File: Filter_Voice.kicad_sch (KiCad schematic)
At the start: 25 parts, among them U3 TL072, U4 SSI2144

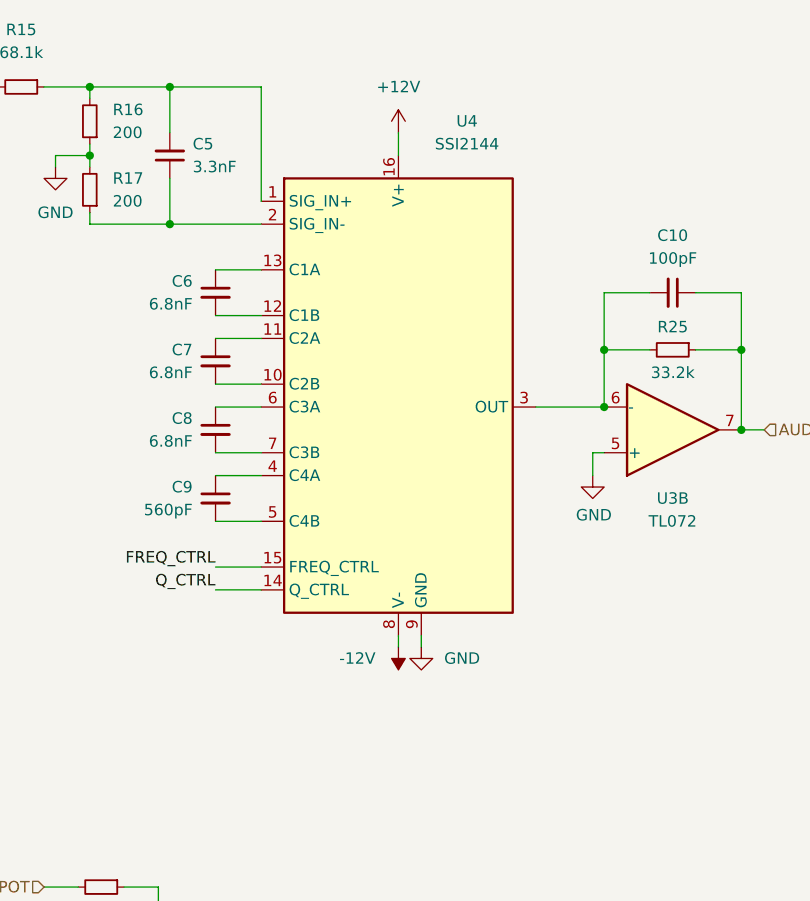
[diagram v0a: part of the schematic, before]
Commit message: First draft of component PCB routed
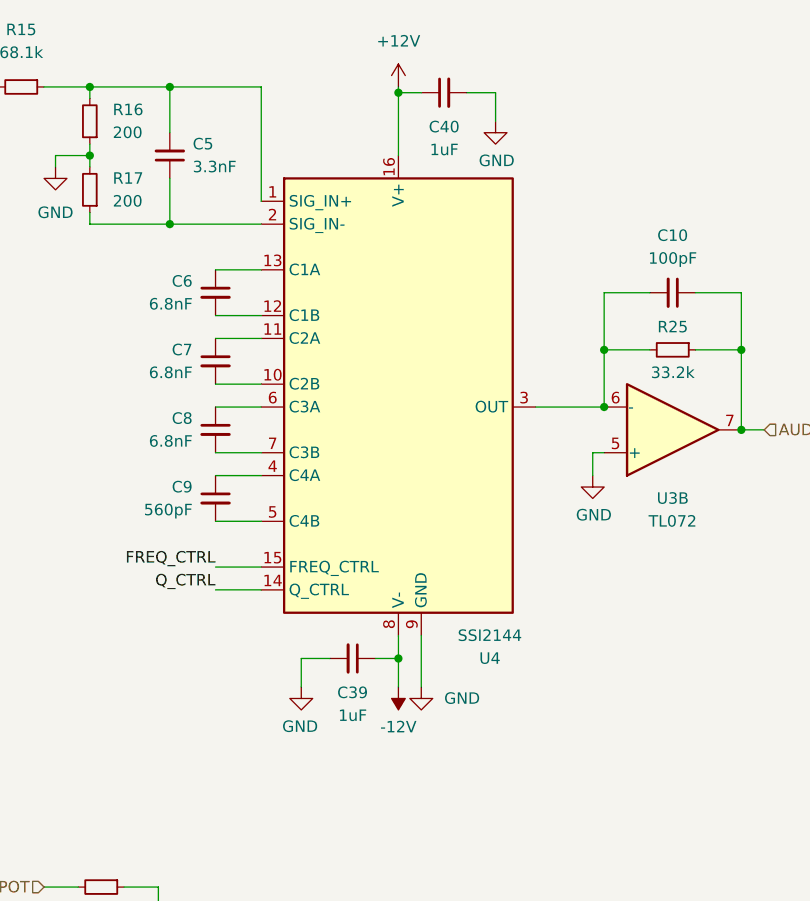
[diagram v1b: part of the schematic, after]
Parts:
- added C39, C40: 1uF, Capacitor_SMD:C_0603_1608Metric_Pad1.08x0.95mm_HandSolder, symbol Device:C_Small
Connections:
- net +12V: now also C40.1
- net -12V: now also C39.1
- net GND: now also C39.2, C40.2
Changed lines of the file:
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@@
   (junction (at 92.71 138.43) (diameter 0) (color 0 0 0 0)
   )
+  (junction (at 80.01 29.845) (diameter 0) (color 0 0 0 0)
+  )
   (junction (at 69.85 128.27) (diameter 0) (color 0 0 0 0)
   )
@@
   (junction (at 158.75 72.39) (diameter 0) (color 0 0 0 0)
   )
+  (junction (at 80.01 92.71) (diameter 0) (color 0 0 0 0)
+  )
   (junction (at 53.34 128.27) (diameter 0) (color 0 0 0 0)
   )
@@
     (stroke (width 0) (type default) (color 0 0 0 0))
   )
+  (wire (pts (xy 82.55 29.845) (xy 80.01 29.845))
+    (stroke (width 0) (type default) (color 0 0 0 0))
+  )
   (wire (pts (xy 45.72 36.83) (xy 45.72 38.1))
     (stroke (width 0) (type default) (color 0 0 0 0))
@@
     (stroke (width 0) (type default) (color 0 0 0 0))
   )
+  (wire (pts (xy 72.39 92.71) (xy 69.215 92.71))
+    (stroke (width 0) (type default) (color 0 0 0 0))
+  )
   (wire (pts (xy 40.64 128.27) (xy 44.45 128.27))
     (stroke (width 0) (type default) (color 0 0 0 0))
@@
     (stroke (width 0) (type default) (color 0 0 0 0))
   )
-  (wire (pts (xy 82.55 91.44) (xy 82.55 90.17))
-    (stroke (width 0) (type default) (color 0 0 0 0))
-  )
-  (wire (pts (xy 80.01 91.44) (xy 80.01 90.17))
+  (wire (pts (xy 82.55 95.885) (xy 82.55 90.17))
+    (stroke (width 0) (type default) (color 0 0 0 0))
+  )
+  (wire (pts (xy 80.01 95.885) (xy 80.01 92.71))
+    (stroke (width 0) (type default) (color 0 0 0 0))
+  )
+  (wire (pts (xy 77.47 92.71) (xy 80.01 92.71))
     (stroke (width 0) (type default) (color 0 0 0 0))
   )
@@
     (stroke (width 0) (type default) (color 0 0 0 0))
   )
+  (wire (pts (xy 90.805 29.845) (xy 90.805 33.02))
+    (stroke (width 0) (type default) (color 0 0 0 0))
+  )
   (wire (pts (xy 66.04 125.73) (xy 66.04 123.19))
     (stroke (width 0) (type default) (color 0 0 0 0))
@@
     (stroke (width 0) (type default) (color 0 0 0 0))
   )
+  (wire (pts (xy 69.215 92.71) (xy 69.215 95.885))
+    (stroke (width 0) (type default) (color 0 0 0 0))
+  )
   (wire (pts (xy 113.03 52.07) (xy 118.11 52.07))
     (stroke (width 0) (type default) (color 0 0 0 0))
@@
     (stroke (width 0) (type default) (color 0 0 0 0))
   )
+  (wire (pts (xy 87.63 29.845) (xy 90.805 29.845))
+    (stroke (width 0) (type default) (color 0 0 0 0))
+  )
   (wire (pts (xy 113.03 58.42) (xy 118.11 58.42))
     (stroke (width 0) (type default) (color 0 0 0 0))
@@
     (stroke (width 0) (type default) (color 0 0 0 0))
   )
+  (wire (pts (xy 80.01 92.71) (xy 80.01 90.17))
+    (stroke (width 0) (type default) (color 0 0 0 0))
+  )
   (wire (pts (xy 158.75 72.39) (xy 161.29 72.39))
     (stroke (width 0) (type default) (color 0 0 0 0))
@@
     (stroke (width 0) (type default) (color 0 0 0 0))
   )
-  (wire (pts (xy 80.01 36.83) (xy 80.01 34.29))
+  (wire (pts (xy 80.01 36.83) (xy 80.01 29.845))
     (stroke (width 0) (type default) (color 0 0 0 0))
   )
@@
   )
   (wire (pts (xy 69.85 128.27) (xy 69.85 138.43))
+    (stroke (width 0) (type default) (color 0 0 0 0))
+  )
+  (wire (pts (xy 80.01 29.845) (xy 80.01 29.21))
     (stroke (width 0) (type default) (color 0 0 0 0))
   )
@@
     (pin "3")
   )
+  (symbol (lib_id "power:GND") (at 69.215 95.885 0) (mirror y) (unit 1)
+    (in_bom yes) (on_board yes)
+    (property "Reference" "#PWR080" (id 0) (at 69.215 102.235 0)
+      (effects (font (size 1.27 1.27)) hide)
+    )
+    (property "Value" "GND" (id 1) (at 69.088 100.2792 0))
+    (property "Footprint" "" (id 2) (at 69.215 95.885 0)
+      (effects (font (size 1.27 1.27)) hide)
+    )
+    (property "Datasheet" "" (id 3) (at 69.215 95.885 0)
+      (effects (font (size 1.27 1.27)) hide)
+    )
+    (pin "1")
+  )
   (symbol (lib_id "Device:R_Small") (at 38.1 29.21 270) (unit 1)
     (in_bom yes) (on_board yes) (fields_autoplaced)
@@
     (pin "2")
   )
+  (symbol (lib_id "Device:C_Small") (at 85.09 29.845 90) (unit 1)
+    (in_bom yes) (on_board yes) (fields_autoplaced)
+    (property "Reference" "C40" (id 0) (at 85.0964 33.655 90))
+    (property "Value" "1uF" (id 1) (at 85.0964 36.195 90))
+    (property "Footprint" "Capacitor_SMD:C_0603_1608Metric_Pad1.08x0.95mm_HandSolder" (id 2) (at 85.09 29.845 0)
+      (effects (font (size 1.27 1.27)) hide)
+    )
+    (property "Datasheet" "~" (id 3) (at 85.09 29.845 0)
+      (effects (font (size 1.27 1.27)) hide)
+    )
+    (pin "1")
+    (pin "2")
+  )
   (symbol (lib_id "power:GND") (at 78.74 148.59 0) (unit 1)
     (in_bom yes) (on_board yes)
@@
     (pin "1")
   )
-  (symbol (lib_id "power:-12V") (at 80.01 91.44 180) (unit 1)
-    (in_bom yes) (on_board yes) (fields_autoplaced)
-    (property "Reference" "#PWR030" (id 0) (at 80.01 93.98 0)
-      (effects (font (size 1.27 1.27)) hide)
-    )
-    (property "Value" "-12V" (id 1) (at 77.47 92.7099 0)
-      (effects (font (size 1.27 1.27)) (justify left))
-    )
-    (property "Footprint" "" (id 2) (at 80.01 91.44 0)
-      (effects (font (size 1.27 1.27)) hide)
-    )
-    (property "Datasheet" "" (id 3) (at 80.01 91.44 0)
+  (symbol (lib_id "power:-12V") (at 80.01 95.885 180) (unit 1)
+    (in_bom yes) (on_board yes) (fields_autoplaced)
+    (property "Reference" "#PWR030" (id 0) (at 80.01 98.425 0)
+      (effects (font (size 1.27 1.27)) hide)
+    )
+    (property "Value" "-12V" (id 1) (at 80.01 100.33 0))
+    (property "Footprint" "" (id 2) (at 80.01 95.885 0)
+      (effects (font (size 1.27 1.27)) hide)
+    )
+    (property "Datasheet" "" (id 3) (at 80.01 95.885 0)
       (effects (font (size 1.27 1.27)) hide)
     )
@@
     (pin "2")
   )
+  (symbol (lib_id "power:GND") (at 90.805 33.02 0) (unit 1)
+    (in_bom yes) (on_board yes)
+    (property "Reference" "#PWR081" (id 0) (at 90.805 39.37 0)
+      (effects (font (size 1.27 1.27)) hide)
+    )
+    (property "Value" "GND" (id 1) (at 90.932 37.4142 0))
+    (property "Footprint" "" (id 2) (at 90.805 33.02 0)
+      (effects (font (size 1.27 1.27)) hide)
+    )
+    (property "Datasheet" "" (id 3) (at 90.805 33.02 0)
+      (effects (font (size 1.27 1.27)) hide)
+    )
+    (pin "1")
+  )
+  (symbol (lib_id "Device:C_Small") (at 74.93 92.71 270) (mirror x) (unit 1)
+    (in_bom yes) (on_board yes) (fields_autoplaced)
+    (property "Reference" "C39" (id 0) (at 74.9236 96.52 90))
+    (property "Value" "1uF" (id 1) (at 74.9236 99.06 90))
+    (property "Footprint" "Capacitor_SMD:C_0603_1608Metric_Pad1.08x0.95mm_HandSolder" (id 2) (at 74.93 92.71 0)
+      (effects (font (size 1.27 1.27)) hide)
+    )
+    (property "Datasheet" "~" (id 3) (at 74.93 92.71 0)
+      (effects (font (size 1.27 1.27)) hide)
+    )
+    (pin "1")
+    (pin "2")
+  )
   (symbol (lib_id "power:+12V") (at 90.17 148.59 90) (unit 1)
     (in_bom yes) (on_board yes)
@@
   (symbol (lib_id "Audio:SSI2144") (at 80.01 64.77 0) (unit 1)
     (in_bom yes) (on_board yes)
-    (property "Reference" "U4" (id 0) (at 87.63 33.02 0))
-    (property "Value" "SSI2144" (id 1) (at 87.63 35.56 0))
+    (property "Reference" "U4" (id 0) (at 90.17 92.71 0))
+    (property "Value" "SSI2144" (id 1) (at 90.17 90.17 0))
     (property "Footprint" "Package_SO:SSOP-16_3.9x4.9mm_P0.635mm" (id 2) (at 102.87 67.31 0)
       (effects (font (size 1.27 1.27)) hide)
@@
     (pin "2")
   )
-  (symbol (lib_id "power:+12V") (at 80.01 34.29 0) (unit 1)
-    (in_bom yes) (on_board yes) (fields_autoplaced)
-    (property "Reference" "#PWR029" (id 0) (at 80.01 38.1 0)
-      (effects (font (size 1.27 1.27)) hide)
-    )
-    (property "Value" "+12V" (id 1) (at 80.01 29.21 0))
-    (property "Footprint" "" (id 2) (at 80.01 34.29 0)
-      (effects (font (size 1.27 1.27)) hide)
-    )
-    (property "Datasheet" "" (id 3) (at 80.01 34.29 0)
-      (effects (font (size 1.27 1.27)) hide)
-    )
-    (pin "1")
-  )
-  (symbol (lib_id "power:GND") (at 82.55 91.44 0) (unit 1)
-    (in_bom yes) (on_board yes) (fields_autoplaced)
-    (property "Reference" "#PWR031" (id 0) (at 82.55 97.79 0)
-      (effects (font (size 1.27 1.27)) hide)
-    )
-    (property "Value" "GND" (id 1) (at 85.09 92.7099 0)
+  (symbol (lib_id "power:+12V") (at 80.01 29.21 0) (unit 1)
+    (in_bom yes) (on_board yes) (fields_autoplaced)
+    (property "Reference" "#PWR029" (id 0) (at 80.01 33.02 0)
+      (effects (font (size 1.27 1.27)) hide)
+    )
+    (property "Value" "+12V" (id 1) (at 80.01 24.13 0))
+    (property "Footprint" "" (id 2) (at 80.01 29.21 0)
+      (effects (font (size 1.27 1.27)) hide)
+    )
+    (property "Datasheet" "" (id 3) (at 80.01 29.21 0)
+      (effects (font (size 1.27 1.27)) hide)
+    )
+    (pin "1")
+  )
+  (symbol (lib_id "power:GND") (at 82.55 95.885 0) (unit 1)
+    (in_bom yes) (on_board yes) (fields_autoplaced)
+    (property "Reference" "#PWR031" (id 0) (at 82.55 102.235 0)
+      (effects (font (size 1.27 1.27)) hide)
+    )
+    (property "Value" "GND" (id 1) (at 85.09 97.1549 0)
       (effects (font (size 1.27 1.27)) (justify left))
     )
-    (property "Footprint" "" (id 2) (at 82.55 91.44 0)
-      (effects (font (size 1.27 1.27)) hide)
-    )
-    (property "Datasheet" "" (id 3) (at 82.55 91.44 0)
-      (effects (font (size 1.27 1.27)) hide)
-    )
+    (property "Footprint" "" (id 2) (at 82.55 95.885 0)
+      (effects (font (size 1.27 1.27)) hide)
+    )
+    (property "Datasheet" "" (id 3) (at 82.55 95.885 0)
+      (effects (font (size 1.27 1.27)) hide)
+    )
